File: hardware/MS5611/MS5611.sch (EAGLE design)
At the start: 4 parts, among them U1 MS5611, U2 EM406FLAT

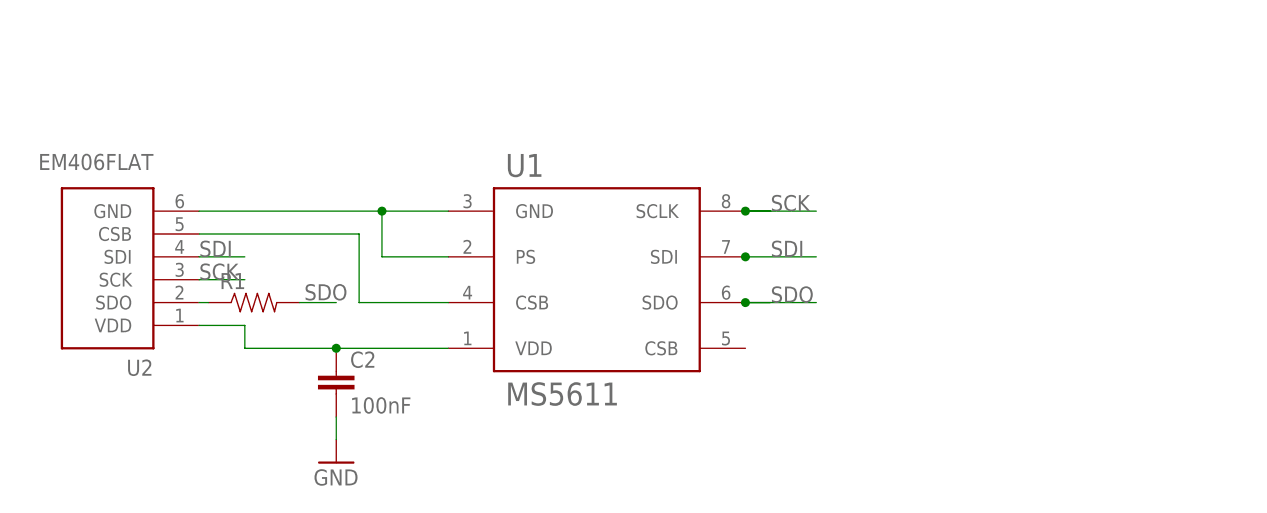
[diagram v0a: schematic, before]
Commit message: MS5611
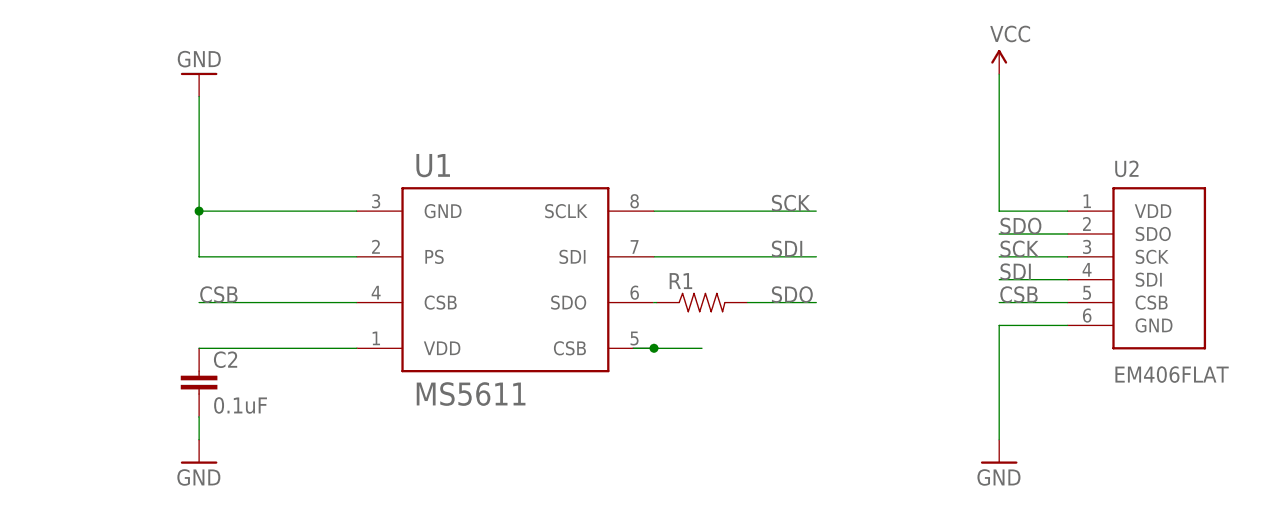
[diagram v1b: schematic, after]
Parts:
- C2: value 100nF -> 0.1uF
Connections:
- net N$6 renamed CSB
- new net N$3: U1.CSB@5
- new net VCC: U2.VDD
- net N$1: now also C2.1, U1.VDD; no longer R1.1, U2.SDO
- net N$2: now also R1.1, U1.SDO; no longer C2.1, U1.VDD, U2.VDD
- net SDO: now also U2.SDO; no longer U1.SDO
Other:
- moved on the sheet: C2, R1, U1, U2
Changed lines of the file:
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@@
 <part name="U2" library="icarus_sensors" deviceset="EM406" device="FLAT"/>
 <part name="GND2" library="icarus_sensors" deviceset="GND" device=""/>
-<part name="C2" library="SparkFun-Capacitors" deviceset="CAP" device="0603-CAP" value="100nF"/>
+<part name="C2" library="SparkFun-Capacitors" deviceset="CAP" device="0603-CAP" value="0.1uF"/>
 <part name="R1" library="SparkFun-Passives" deviceset="RESISTOR" device="0603-RES"/>
+<part name="GND1" library="icarus_sensors" deviceset="GND" device=""/>
+<part name="GND3" library="icarus_sensors" deviceset="GND" device=""/>
+<part name="SUPPLY1" library="icarus_sensors" deviceset="VCC" device=""/>
 </parts>
 <sheets>
@@
 </plain>
 <instances>
-<instance part="U1" gate="G$1" x="1.016" y="-2.54"/>
-<instance part="U2" gate="G$1" x="-53.34" y="-2.54" rot="R180"/>
-<instance part="GND2" gate="1" x="-25.4" y="-22.86"/>
-<instance part="C2" gate="G$1" x="-25.4" y="-15.24"/>
-<instance part="R1" gate="G$1" x="-34.544" y="-5.08"/>
+<instance part="U1" gate="G$1" x="-9.144" y="-2.54"/>
+<instance part="U2" gate="G$1" x="68.58" y="0"/>
+<instance part="GND2" gate="1" x="-40.64" y="-22.86"/>
+<instance part="C2" gate="G$1" x="-40.64" y="-15.24"/>
+<instance part="R1" gate="G$1" x="15.24" y="-5.08"/>
+<instance part="GND1" gate="1" x="48.26" y="-22.86"/>
+<instance part="GND3" gate="1" x="-40.64" y="20.32" rot="R180"/>
+<instance part="SUPPLY1" gate="G$1" x="48.26" y="20.32"/>
 </instances>
 <busses>
 </busses>
 <nets>
-<net name="N$6" class="0">
-<segment>
-<pinref part="U2" gate="G$1" pin="CSB"/>
-<wire x1="-40.64" y1="2.54" x2="-22.86" y2="2.54" width="0.1524" layer="91"/>
-<wire x1="-22.86" y1="2.54" x2="-22.86" y2="-5.08" width="0.1524" layer="91"/>
-<wire x1="-22.86" y1="-5.08" x2="-12.954" y2="-5.08" width="0.1524" layer="91"/>
-<pinref part="U1" gate="G$1" pin="CSB@4"/>
-</segment>
-</net>
 <net name="SCK" class="0">
 <segment>
-<pinref part="U2" gate="G$1" pin="SCK"/>
-<wire x1="-40.64" y1="-2.54" x2="-35.56" y2="-2.54" width="0.1524" layer="91"/>
-<label x="-40.64" y="-2.54" size="1.778" layer="95"/>
+<pinref part="U1" gate="G$1" pin="SCLK"/>
+<wire x1="9.906" y1="5.08" x2="27.94" y2="5.08" width="0.1524" layer="91"/>
+<label x="22.86" y="5.08" size="1.778" layer="95"/>
 </segment>
 <segment>
-<wire x1="22.86" y1="5.08" x2="20.066" y2="5.08" width="0.1524" layer="91"/>
-<pinref part="U1" gate="G$1" pin="SCLK"/>
-<wire x1="20.066" y1="5.08" x2="27.94" y2="5.08" width="0.1524" layer="91"/>
-<junction x="20.066" y="5.08"/>
-<label x="22.86" y="5.08" size="1.778" layer="95"/>
+<pinref part="U2" gate="G$1" pin="SCK"/>
+<wire x1="55.88" y1="0" x2="48.26" y2="0" width="0.1524" layer="91"/>
+<label x="48.26" y="0" size="1.778" layer="95"/>
 </segment>
 </net>
 <net name="SDI" class="0">
 <segment>
-<pinref part="U2" gate="G$1" pin="SDI"/>
-<wire x1="-40.64" y1="0" x2="-35.56" y2="0" width="0.1524" layer="91"/>
-<label x="-40.64" y="0" size="1.778" layer="95"/>
+<pinref part="U1" gate="G$1" pin="SDI"/>
+<wire x1="9.906" y1="0" x2="27.94" y2="0" width="0.1524" layer="91"/>
+<label x="22.86" y="0" size="1.778" layer="95"/>
 </segment>
 <segment>
-<wire x1="20.32" y1="0" x2="20.066" y2="0" width="0.1524" layer="91"/>
-<pinref part="U1" gate="G$1" pin="SDI"/>
-<wire x1="20.066" y1="0" x2="27.94" y2="0" width="0.1524" layer="91"/>
-<junction x="20.066" y="0"/>
-<label x="22.86" y="0" size="1.778" layer="95"/>
-</segment>
-</net>
-<net name="SDO" class="0">
-<segment>
-<wire x1="22.86" y1="-5.08" x2="20.066" y2="-5.08" width="0.1524" layer="91"/>
-<pinref part="U1" gate="G$1" pin="SDO"/>
-<wire x1="20.066" y1="-5.08" x2="27.94" y2="-5.08" width="0.1524" layer="91"/>
-<junction x="20.066" y="-5.08"/>
-<label x="22.86" y="-5.08" size="1.778" layer="95"/>
-</segment>
-<segment>
-<pinref part="R1" gate="G$1" pin="2"/>
-<wire x1="-29.464" y1="-5.08" x2="-25.4" y2="-5.08" width="0.1524" layer="91"/>
-<label x="-28.956" y="-4.826" size="1.778" layer="95"/>
-</segment>
-</net>
-<net name="N$2" class="0">
-<segment>
-<pinref part="U2" gate="G$1" pin="VDD"/>
-<wire x1="-40.64" y1="-7.62" x2="-35.56" y2="-7.62" width="0.1524" layer="91"/>
-<wire x1="-35.56" y1="-7.62" x2="-35.56" y2="-10.16" width="0.1524" layer="91"/>
-<pinref part="U1" gate="G$1" pin="VDD"/>
-<wire x1="-35.56" y1="-10.16" x2="-25.4" y2="-10.16" width="0.1524" layer="91"/>
-<pinref part="C2" gate="G$1" pin="1"/>
-<wire x1="-25.4" y1="-10.16" x2="-12.954" y2="-10.16" width="0.1524" layer="91"/>
-<junction x="-25.4" y="-10.16"/>
+<pinref part="U2" gate="G$1" pin="SDI"/>
+<wire x1="55.88" y1="-2.54" x2="48.26" y2="-2.54" width="0.1524" layer="91"/>
+<label x="48.26" y="-2.54" size="1.778" layer="95"/>
 </segment>
 </net>
@@
 <pinref part="C2" gate="G$1" pin="2"/>
 <pinref part="GND2" gate="1" pin="GND"/>
-<wire x1="-25.4" y1="-17.78" x2="-25.4" y2="-20.32" width="0.1524" layer="91"/>
+<wire x1="-40.64" y1="-17.78" x2="-40.64" y2="-20.32" width="0.1524" layer="91"/>
 </segment>
 <segment>
 <pinref part="U2" gate="G$1" pin="GND"/>
-<wire x1="-20.32" y1="5.08" x2="-40.64" y2="5.08" width="0.1524" layer="91"/>
-<wire x1="-20.32" y1="0" x2="-20.32" y2="5.08" width="0.1524" layer="91"/>
+<pinref part="GND1" gate="1" pin="GND"/>
+<wire x1="55.88" y1="-7.62" x2="48.26" y2="-7.62" width="0.1524" layer="91"/>
+<wire x1="48.26" y1="-7.62" x2="48.26" y2="-20.32" width="0.1524" layer="91"/>
+</segment>
+<segment>
+<pinref part="GND3" gate="1" pin="GND"/>
+<wire x1="-23.114" y1="5.08" x2="-40.64" y2="5.08" width="0.1524" layer="91"/>
+<wire x1="-40.64" y1="5.08" x2="-40.64" y2="17.78" width="0.1524" layer="91"/>
+<wire x1="-23.114" y1="0" x2="-40.64" y2="0" width="0.1524" layer="91"/>
+<wire x1="-40.64" y1="0" x2="-40.64" y2="5.08" width="0.1524" layer="91"/>
+<junction x="-40.64" y="5.08"/>
 <pinref part="U1" gate="G$1" pin="GND"/>
-<wire x1="-20.32" y1="5.08" x2="-12.954" y2="5.08" width="0.1524" layer="91"/>
-<junction x="-20.32" y="5.08"/>
 <pinref part="U1" gate="G$1" pin="PS"/>
-<wire x1="-12.954" y1="0" x2="-20.32" y2="0" width="0.1524" layer="91"/>
 </segment>
 </net>
 <net name="N$1" class="0">
 <segment>
-<pinref part="U2" gate="G$1" pin="SDO"/>
-<pinref part="R1" gate="G$1" pin="1"/>
-<wire x1="-40.64" y1="-5.08" x2="-39.624" y2="-5.08" width="0.1524" layer="91"/>
+<pinref part="U1" gate="G$1" pin="VDD"/>
+<pinref part="C2" gate="G$1" pin="1"/>
+<wire x1="-40.64" y1="-10.16" x2="-23.114" y2="-10.16" width="0.1524" layer="91"/>
 </segment>
 </net>
+<net name="VCC" class="0">
+<segment>
+<pinref part="U2" gate="G$1" pin="VDD"/>
+<pinref part="SUPPLY1" gate="G$1" pin="VCC"/>
+<wire x1="55.88" y1="5.08" x2="48.26" y2="5.08" width="0.1524" layer="91"/>
+<wire x1="48.26" y1="5.08" x2="48.26" y2="20.32" width="0.1524" layer="91"/>
+</segment>
+</net>
+<net name="SDO" class="0">
+<segment>
+<wire x1="20.32" y1="-5.08" x2="27.94" y2="-5.08" width="0.1524" layer="91"/>
+<label x="22.86" y="-5.08" size="1.778" layer="95"/>
+<pinref part="R1" gate="G$1" pin="2"/>
+</segment>
+<segment>
+<label x="48.26" y="2.54" size="1.778" layer="95"/>
+<pinref part="U2" gate="G$1" pin="SDO"/>
+<wire x1="55.88" y1="2.54" x2="48.26" y2="2.54" width="0.1524" layer="91"/>
+</segment>
+</net>
+<net name="CSB" class="0">
+<segment>
+<pinref part="U2" gate="G$1" pin="CSB"/>
+<wire x1="55.88" y1="-5.08" x2="48.26" y2="-5.08" width="0.1524" layer="91"/>
+<label x="48.26" y="-5.08" size="1.778" layer="95"/>
+</segment>
+<segment>
+<wire x1="-40.64" y1="-5.08" x2="-23.114" y2="-5.08" width="0.1524" layer="91"/>
+<pinref part="U1" gate="G$1" pin="CSB@4"/>
+<label x="-40.64" y="-5.08" size="1.778" layer="95"/>
+</segment>
+</net>
+<net name="N$2" class="0">
+<segment>
+<wire x1="10.16" y1="-5.08" x2="9.906" y2="-5.08" width="0.1524" layer="91"/>
+<pinref part="R1" gate="G$1" pin="1"/>
+<pinref part="U1" gate="G$1" pin="SDO"/>
+</segment>
+</net>
+<net name="N$3" class="0">
+<segment>
+<wire x1="7.62" y1="-10.16" x2="9.906" y2="-10.16" width="0.1524" layer="91"/>
+<pinref part="U1" gate="G$1" pin="CSB@5"/>
+<wire x1="9.906" y1="-10.16" x2="15.24" y2="-10.16" width="0.1524" layer="91"/>
+<junction x="9.906" y="-10.16"/>
+</segment>
+</net>
